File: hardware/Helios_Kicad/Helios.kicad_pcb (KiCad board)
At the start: 2 copper layers, 75 x 61 mm, 95 parts, among them P1 USB_B, P2 CONN_01X25-SHIELD, P3 CONN_01X03, U1 IP4220CZ6, U2 AP2114, U3 AN431B, U4 ISA_DC-DC_converter, U5 DAC084S085C, U6 TL084_v, U7 LM358, U8 TL084_v, U9 ATSAM4S, Y1 16MHz 18pF

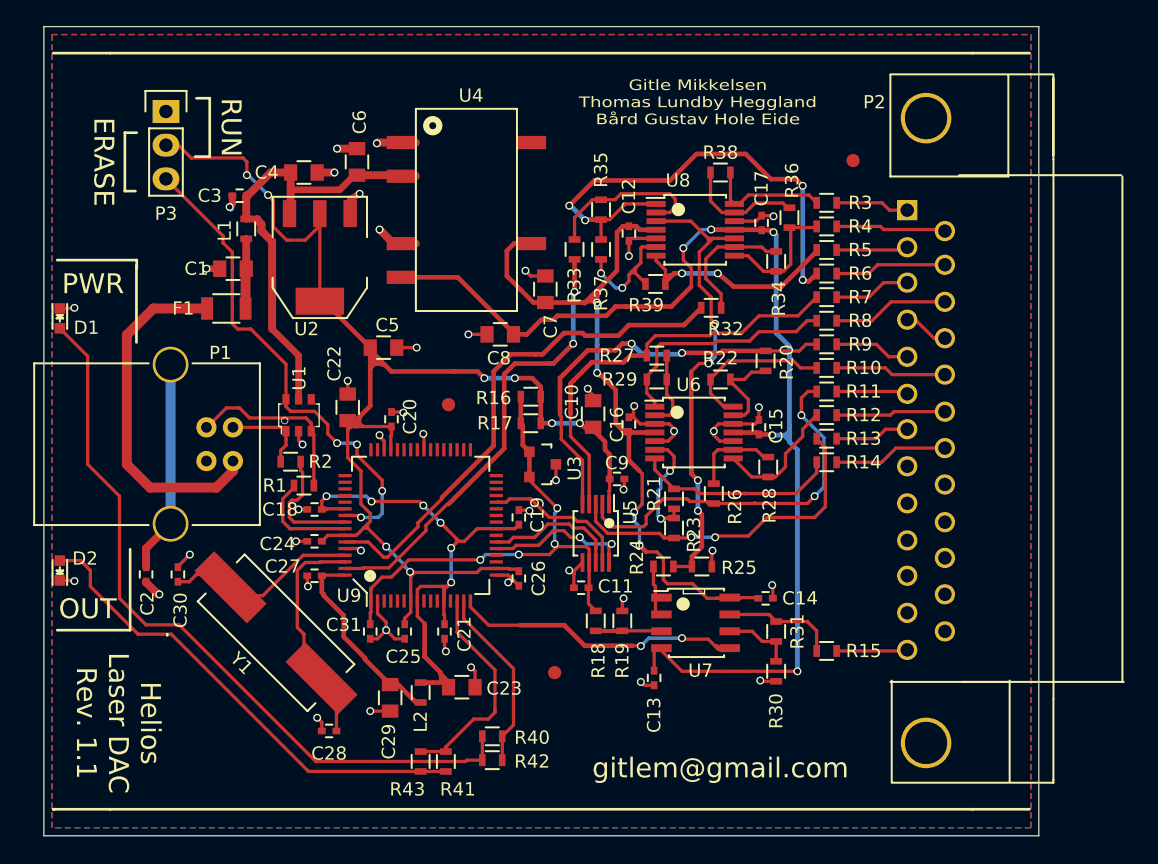
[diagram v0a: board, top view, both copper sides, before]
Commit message: redone pcb, driver and firmware working-ish
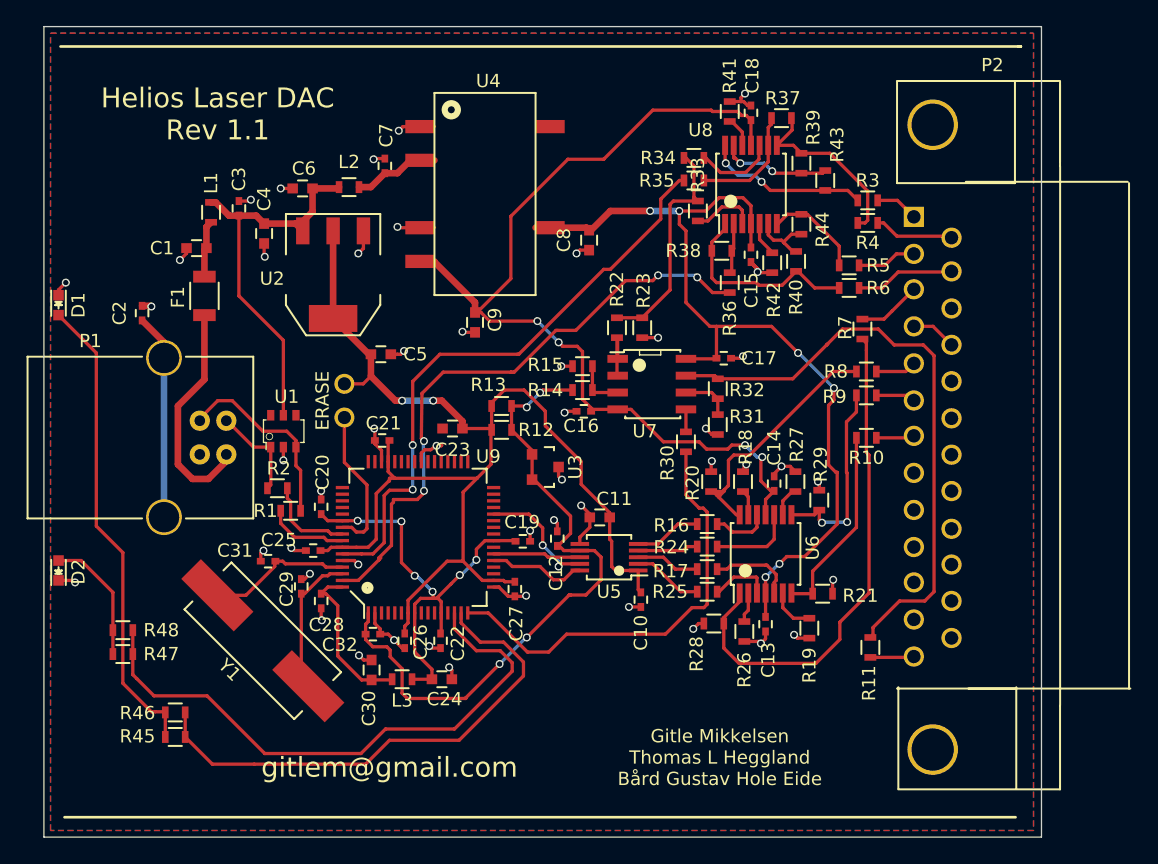
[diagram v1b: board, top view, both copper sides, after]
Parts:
- removed ? (x3): Fiducial_1mm_Dia_2.54mm_Outer_CopperTop, Fiducials:Fiducial_1mm_Dia_2.54mm_Outer_CopperTop
- removed P3: CONN_01X03, Pin_Headers:Pin_Header_Straight_1x03
- added C32: 13pF, Capacitors_SMD:C_0402, F.Cu at (124.8, 145.8)
- added ERASE: CONN_01X02, Connect:PINHEAD1-2, F.Cu at (122.7, 128.2)
- added L3: FILTER, Resistors_SMD:R_0603, F.Cu at (127.0, 149.2)
- added R44: 10k, Resistors_SMD:R_0603, F.Cu at (157.1, 114.9)
- added R45: 1.65k, Resistors_SMD:R_0603, F.Cu at (109.9, 153.6)
- added R46: 1.65k, Resistors_SMD:R_0603, F.Cu at (109.9, 151.7)
- added R47: 1.65k, Resistors_SMD:R_0603, F.Cu at (106.0, 147.3)
- added R48: 1.65k, Resistors_SMD:R_0603, F.Cu at (106.0, 145.5)
- C1, C23, C4, C5, C6, C8: footprint Capacitors_SMD:C_0805 -> Capacitors_SMD:C_0603
- C10, C22, C7: value 4.7uF -> 100nF; footprint Capacitors_SMD:C_0805 -> Capacitors_SMD:C_0402
- C11, C30: value 13pF -> 4.7uF; footprint Capacitors_SMD:C_0402 -> Capacitors_SMD:C_0603
- C12: value 100nF -> 13pF
- C24, C9: value 100nF -> 4.7uF; footprint Capacitors_SMD:C_0402 -> Capacitors_SMD:C_0603
- C28: value 13pF -> 100nF
- C29: value 4.7uF -> 13pF; footprint Capacitors_SMD:C_0805 -> Capacitors_SMD:C_0402
- F1: value PTC -> F_Small
- L1, L2: value FERRITE_BEAD -> FILTER
- R14, R15: value 150 -> 10k
- R16, R17: value 150 -> 5.11k
- R22, R34, R35, R36: value 10k -> 1.65k
- R24, R32, R41, R42: value 1.65k -> 5.11k
- R25, R30: value 10k -> 5.11k
- R31: value 5.11k -> 10k
- R40, R43: value 1.65k -> 10k
- U2: footprint SOT-223 -> TO_SOT_Packages_SMD:SOT-223
- U7: footprint SOIC-8_3.9x4.9mm_Pitch1.27mm -> personal:SOIC-8_3.9x4.9mm_Pitch1.27mm
- moved R41 53.5 mm to (151.7, 106.4), turned to 90 degrees
- moved R43 53.4 mm to (158.9, 111.6), turned to 90 degrees
- moved C18 44.5 mm to (153.3, 106.5), turned to 270 degrees
- moved R42 43.0 mm to (154.9, 117.8), turned to 270 degrees
- moved R40 42.5 mm to (156.7, 117.7), turned to 270 degrees
- moved L2 38.5 mm to (123.0, 112.1), turned to 0 degrees
- moved R15 28.3 mm to (140.6, 125.6)
- moved R13 24.6 mm to (134.5, 128.6), turned to 0 degrees
- moved R12 24.5 mm to (134.5, 130.4), turned to 0 degrees
- moved C12 23.6 mm to (138.7, 138.6), turned to 270 degrees
- moved C2 19.7 mm to (107.4, 121.6), turned to 90 degrees
- moved R11 19.6 mm to (162.3, 146.8), turned to 90 degrees
- moved C23 19.5 mm to (130.8, 130.3), turned to 180 degrees
- moved R14 19.2 mm to (140.6, 127.4), turned to 0 degrees
- moved C22 18.9 mm to (129.9, 146.3), turned to 270 degrees
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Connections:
- C11 pad 1: GND -> /DAC/3.3V
- C11 pad 2: /Amplifiers/2.5V -> GND
- C12 pad 2: /Amplifiers/+9V -> /Amplifiers/2.5V
- C13 pad 2: /Amplifiers/-9V -> /Amplifiers/+9V
- C14 pad 2: /Amplifiers/+9V -> /Amplifiers/-9V
- C15 pad 2: /Amplifiers/-9V -> /Amplifiers/+9V
- C16 pad 2: /Amplifiers/+9V -> /Amplifiers/-9V
- C17 pad 2: /Amplifiers/-9V -> /Amplifiers/+9V
- C18 pad 1: /Microcontroller/VDDOUT -> GND
- C18 pad 2: GND -> /Amplifiers/-9V
- C20 pad 1: /DAC/3.3V -> /Microcontroller/VDDOUT
- C21 pad 1: /Microcontroller/VDDOUT -> /DAC/3.3V
- C22 pad 1: /DAC/3.3V -> /Microcontroller/VDDOUT
- C23 pad 1: /Microcontroller/VDDOUT -> /DAC/3.3V
- C24 pad 1: /DAC/3.3V -> /Microcontroller/VDDOUT
- C27 pad 1: /Microcontroller/VDDPLL -> /DAC/3.3V
- C28 pad 1: /Microcontroller/XIN -> /Microcontroller/VDDPLL
- C29 pad 1: /Microcontroller/VDDPLL -> /Microcontroller/XIN
- C30 pad 1: /Microcontroller/XOUT -> /Microcontroller/VDDPLL
- C31 pad 1: /Amplifiers/2.5V -> /Microcontroller/XOUT
- C7 pad 1: GND -> Net-(C7-Pad1)
- C7 pad 2: /Amplifiers/+9V -> GND
- C8 pad 1: /Amplifiers/-9V -> GND
- C8 pad 2: GND -> /Amplifiers/+9V
- C9 pad 1: /DAC/3.3V -> /Amplifiers/-9V
- L2 pad 1: /Microcontroller/VDDOUT -> /Power Regulation/5V
- L2 pad 2: /Microcontroller/VDDPLL -> Net-(C7-Pad1)
- P2 pad 16: Net-(P2-Pad16) -> GND
- P2 pad 18: Net-(P2-Pad18) -> GND
- P2 pad 19: Net-(P2-Pad19) -> GND
- P2 pad 20: Net-(P2-Pad20) -> GND
- R10 pad 1: Net-(P2-Pad18) -> Net-(P2-Pad7)
- R10 pad 2: /Amplifiers/-R -> /Amplifiers/+B
- R11 pad 1: Net-(P2-Pad6) -> Net-(P2-Pad13)
- R11 pad 2: /Amplifiers/+G -> /Amplifiers/Shutter_Out
- R12 pad 1: Net-(P2-Pad19) -> /DAC/3.3V
- R12 pad 2: /Amplifiers/-G -> /Amplifiers/2.5V
- R13 pad 1: Net-(P2-Pad7) -> /DAC/3.3V
- R13 pad 2: /Amplifiers/+B -> /Amplifiers/2.5V
- R14 pad 1: Net-(P2-Pad20) -> /Amplifiers/2.5V
- R14 pad 2: /Amplifiers/-B -> Net-(R14-Pad2)
- R15 pad 1: Net-(P2-Pad13) -> Net-(R14-Pad2)
- R15 pad 2: /Amplifiers/Shutter_Out -> GND
- R16 pad 1: /DAC/3.3V -> Net-(R16-Pad1)
- R16 pad 2: /Amplifiers/2.5V -> /Amplifiers/R
- R17 pad 1: /DAC/3.3V -> Net-(R17-Pad1)
- R17 pad 2: /Amplifiers/2.5V -> /Amplifiers/B
- R18 pad 1: /Amplifiers/2.5V -> GND
- R19 pad 1: Net-(R18-Pad2) -> GND
- R19 pad 2: GND -> Net-(R19-Pad2)
- R20 pad 1: Net-(R20-Pad1) -> /Amplifiers/+R
- R20 pad 2: /Amplifiers/+R -> GND
- R21 pad 1: Net-(R21-Pad1) -> /Amplifiers/+B
- R21 pad 2: /Amplifiers/+B -> GND
- R22 pad 1: /Amplifiers/-R -> Net-(R22-Pad1)
- R22 pad 2: Net-(R20-Pad1) -> /Amplifiers/Offset
- R23 pad 1: /Amplifiers/-B -> /Amplifiers/Offset
- R23 pad 2: Net-(R21-Pad1) -> GND
- R24 pad 2: /Amplifiers/Offset -> /Amplifiers/G
- R25 pad 1: /Amplifiers/Offset -> Net-(R25-Pad1)
- R25 pad 2: GND -> /Amplifiers/Intensity
- R26 pad 1: Net-(R26-Pad1) -> GND
- R26 pad 2: /Amplifiers/+G -> Net-(R26-Pad2)
- R27 pad 1: Net-(R27-Pad1) -> GND
- R27 pad 2: /Amplifiers/+Intensity -> Net-(R27-Pad2)
- R28 pad 1: /Amplifiers/-G -> /Amplifiers/+Intensity
- R28 pad 2: Net-(R26-Pad1) -> GND
- R29 pad 1: /Amplifiers/-Intensity -> /Amplifiers/+G
- R29 pad 2: Net-(R27-Pad1) -> GND
- R30 pad 1: GND -> Net-(R30-Pad1)
- R30 pad 2: Net-(R30-Pad2) -> /Amplifiers/Shutter
- R31 pad 1: /Amplifiers/Shutter_Out -> GND
- R31 pad 2: Net-(R30-Pad2) -> Net-(R31-Pad2)
- R32 pad 1: Net-(R32-Pad1) -> /Amplifiers/Shutter_Out
- R32 pad 2: /Amplifiers/X -> Net-(R31-Pad2)
- R33 pad 2: /Amplifiers/Y -> /Amplifiers/Offset
- R34 pad 1: /Amplifiers/-X -> Net-(R34-Pad1)
- R34 pad 2: Net-(R32-Pad1) -> /Amplifiers/Offset
- R35 pad 1: /Amplifiers/-Y -> Net-(R35-Pad1)
- R35 pad 2: Net-(R33-Pad1) -> /Amplifiers/X
- R36 pad 2: /Amplifiers/-X -> /Amplifiers/Y
- R37 pad 1: Net-(R37-Pad1) -> /Amplifiers/-X
- R37 pad 2: /Amplifiers/-Y -> Net-(R35-Pad1)
- R38 pad 1: /Amplifiers/+X -> /Amplifiers/-Y
- R39 pad 1: /Amplifiers/+Y -> Net-(R39-Pad1)
- R39 pad 2: Net-(R37-Pad1) -> /Amplifiers/-X
- R40 pad 1: /Microcontroller/PA23 -> Net-(R40-Pad1)
- R40 pad 2: Net-(D1-Pad2) -> /Amplifiers/-Y
- R41 pad 1: /Microcontroller/PA22 -> Net-(R41-Pad1)
- R41 pad 2: Net-(D2-Pad2) -> GND
- R42 pad 1: /Microcontroller/PA23 -> Net-(R42-Pad1)
- R42 pad 2: Net-(D1-Pad2) -> GND
- R43 pad 1: /Microcontroller/PA22 -> /Amplifiers/+X
- R43 pad 2: Net-(D2-Pad2) -> Net-(R39-Pad1)
- R8 pad 1: Net-(P2-Pad16) -> Net-(P2-Pad5)
- R8 pad 2: /Amplifiers/-Intensity -> /Amplifiers/+R
- R9 pad 1: Net-(P2-Pad5) -> Net-(P2-Pad6)
- R9 pad 2: /Amplifiers/+R -> /Amplifiers/+G
- U1 pad 6: /Microcontroller/ERASE -> (no net)
- U4 pad 2: /Power Regulation/5V -> Net-(C7-Pad1)
- U5 pad 2: /Amplifiers/+G -> /Amplifiers/Intensity
- U5 pad 3: /Amplifiers/+B -> /Amplifiers/B
- U5 pad 4: /Amplifiers/+Intensity -> /Amplifiers/G
- U5 pad 5: /Amplifiers/+R -> /Amplifiers/R
- U6 pad 1: /Amplifiers/-Intensity -> /Amplifiers/+Intensity
- U6 pad 10: GND -> Net-(R24-Pad1)
- U6 pad 12: GND -> Net-(R16-Pad1)
- U6 pad 13: Net-(R20-Pad1) -> Net-(R18-Pad2)
- U6 pad 14: /Amplifiers/-R -> /Amplifiers/+R
- U6 pad 2: Net-(R27-Pad1) -> Net-(R26-Pad2)
- U6 pad 3: GND -> Net-(R25-Pad1)
- U6 pad 5: GND -> Net-(R17-Pad1)
- U6 pad 6: Net-(R21-Pad1) -> Net-(R19-Pad2)
- U6 pad 7: /Amplifiers/-B -> /Amplifiers/+B
- U6 pad 8: /Amplifiers/-G -> /Amplifiers/+G
- U6 pad 9: Net-(R26-Pad1) -> Net-(R27-Pad2)
- U7 pad 1: Net-(R24-Pad1) -> Net-(R22-Pad1)
- U7 pad 2: Net-(R24-Pad1) -> Net-(R22-Pad1)
- U7 pad 3: Net-(R18-Pad2) -> Net-(R14-Pad2)
- U7 pad 5: /Amplifiers/Shutter -> Net-(R30-Pad1)
- U7 pad 6: Net-(R30-Pad2) -> Net-(R31-Pad2)
- U8 pad 10: /Amplifiers/Offset -> Net-(R34-Pad1)
- U8 pad 12: GND -> Net-(R41-Pad1)
- U8 pad 13: Net-(R36-Pad1) -> Net-(R39-Pad1)
- U8 pad 2: Net-(R33-Pad1) -> Net-(R36-Pad1)
- U8 pad 3: /Amplifiers/Offset -> Net-(R33-Pad1)
- U8 pad 5: GND -> Net-(R42-Pad1)
- U8 pad 6: Net-(R37-Pad1) -> Net-(R40-Pad1)
- U8 pad 9: Net-(R32-Pad1) -> Net-(R35-Pad1)
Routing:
- net /Amplifiers/Shutter_Out: track 8.93 -> 45.7 mm
- net /Microcontroller/PA22: track 16.6 -> 44.2 mm
- net Net-(D2-Pad2): track 36.4 -> 9.74 mm
- net /Microcontroller/ERASE: track 37.5 -> 11.2 mm, vias 4 -> 0
- net /Microcontroller/PA23: track 13.9 -> 38.7 mm
- net /Amplifiers/-Y: track 37.7 -> 15.3 mm, vias 4 -> 0
- net Net-(D1-Pad2): track 56.5 -> 35.7 mm
- net /Amplifiers/Offset: track 35.6 -> 17.3 mm, vias 4 -> 0
- net /DAC/3.3V: track 111.2 -> 92.9 mm, vias 8 -> 2
- net /Amplifiers/-Intensity: track 17.9 -> 0.00 mm
- net /Amplifiers/-9V: track 87.9 -> 71.2 mm, vias 5 -> 4
- net /Amplifiers/-B: track 15.4 -> 0.00 mm
- net /Amplifiers/+G: track 29.0 -> 15.1 mm
- net /Amplifiers/2.5V: track 38.4 -> 50.6 mm
- net /Amplifiers/Y: track 34.1 -> 46.2 mm, vias 2 -> 4
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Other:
- board size 75 x 61 mm -> 75.2 x 61.1 mm
- net class Power removed
- board text added: "Gitle Mikkelsen Thomas L Heggland Bård Gustav Hole Eide"
- board text added: "Helios Laser DAC Rev 1.1"
- board text removed: "ERASE"
- board text removed: "Gitle Mikkelsen Thomas Lundby Heggland Bård Gustav Hole Eide"
- board text removed: "Helios Laser DAC Rev. 1.1"
- board text removed: "OUT"
- board text removed: "PWR"
- board text removed: "RUN"
